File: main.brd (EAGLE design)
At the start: 36.8 x 28.6 mm, 22 parts, among them Y1 16MHz

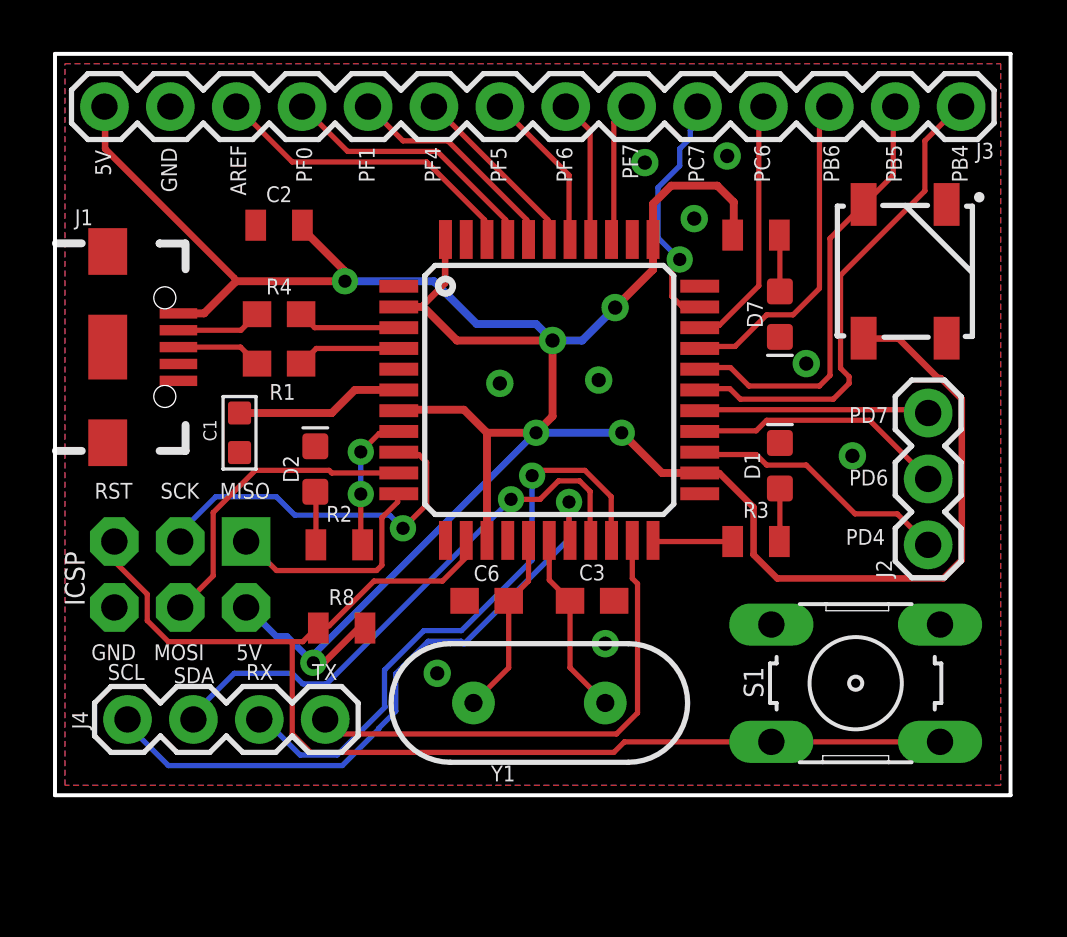
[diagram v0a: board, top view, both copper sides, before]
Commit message: Gerber file re process
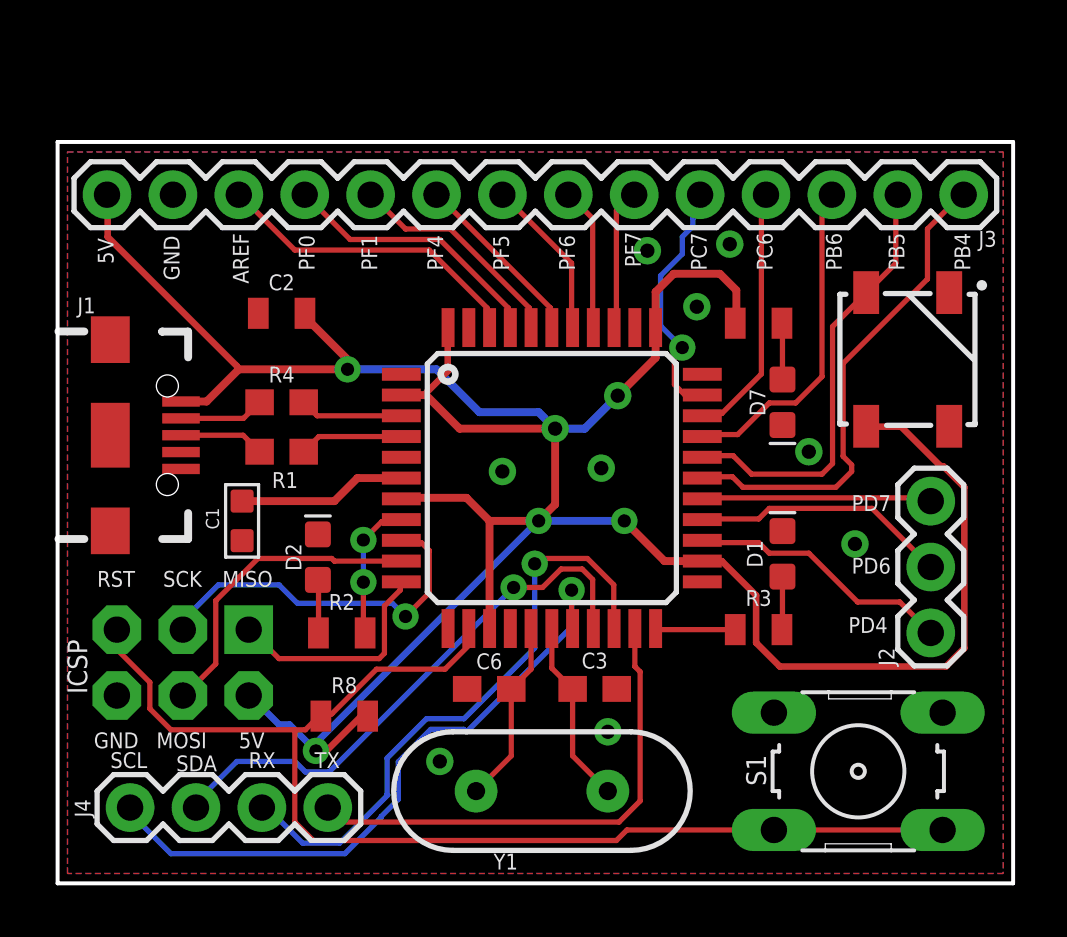
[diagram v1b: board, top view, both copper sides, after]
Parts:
- moved C1 3.40 mm to (7.21, 14.0)
- moved C3 3.40 mm to (20.8, 7.53)
- moved C6 3.40 mm to (16.7, 7.53)
- moved D1 3.40 mm to (28.0, 12.7)
- moved D3 3.40 mm to (32.9, 20.2)
- moved D7 3.40 mm to (28.0, 18.6)
- moved ICSP 3.40 mm to (4.93, 8.54)
- moved J1 3.40 mm to (2.13, 17.3)
- moved J3 3.40 mm to (35.0, 26.6)
- moved R1 3.40 mm to (8.74, 16.7)
- moved R3 3.40 mm to (27.1, 9.81)
- moved R4 3.40 mm to (8.74, 18.6)
- moved U$1 3.40 mm to (19.1, 15.7)
- moved Y1 3.40 mm to (18.8, 3.59)
- moved J4 3.40 mm to (2.89, 2.95)
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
